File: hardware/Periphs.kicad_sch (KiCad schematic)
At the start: 0 parts

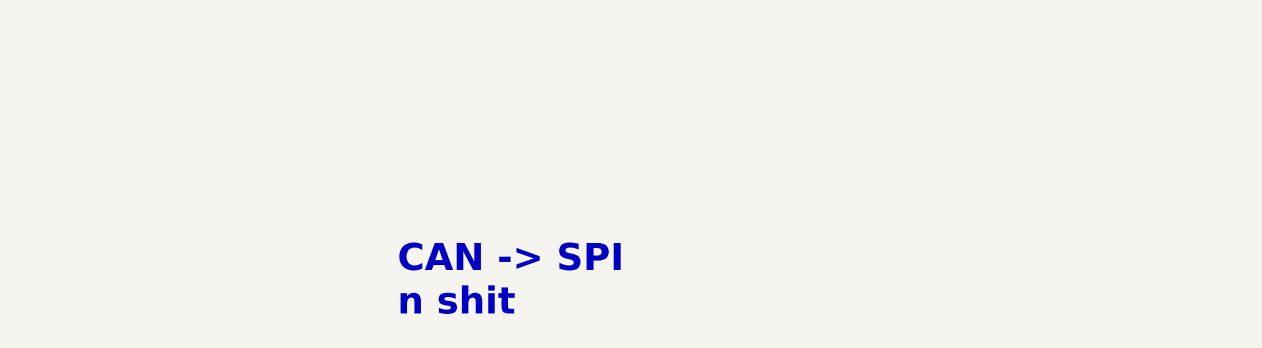
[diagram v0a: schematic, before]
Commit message: poop
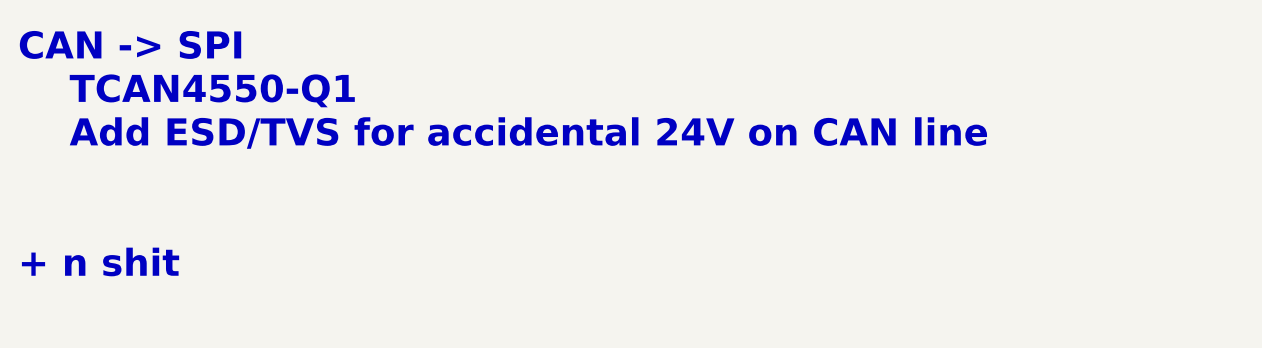
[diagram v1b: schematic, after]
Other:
- note added: "CAN -> SPI TCAN4550-Q1 Add ESD/TVS for accidental 24V on CAN line + n shit"
- note removed: "CAN -> SPI n shit"
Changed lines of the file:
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@@
 	(generator_version "10.0")
 	(paper "A4")
-	(text "CAN -> SPI\nn shit"
+	(text "CAN -> SPI\n	TCAN4550-Q1\n	Add ESD/TVS for accidental 24V on CAN line\n\n\n+ n shit\n	"
 		(exclude_from_sim no)
-		(at 129.032 96.52 0)
+		(at 86.868 85.09 0)
 		(effects
 			(font
